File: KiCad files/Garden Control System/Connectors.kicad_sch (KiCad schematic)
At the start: 8 parts, among them J2 PJ-102AH, J3 Debug, J4 USB_C_Receptacle_USB2.0, J5 PJ-102AH, J6 PJ-102AH, J7 PJ-102AH

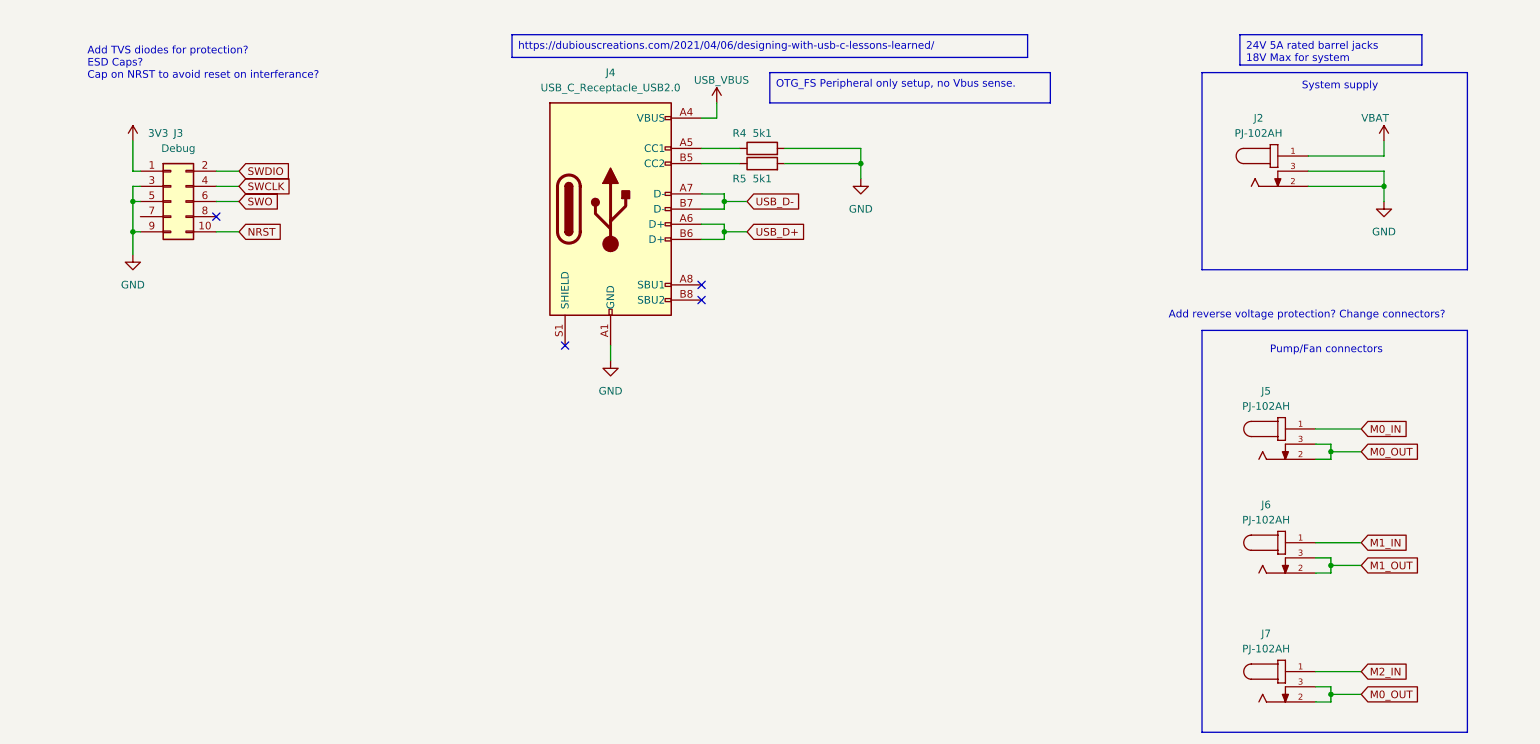
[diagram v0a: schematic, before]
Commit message: we cookin' again. Added LSD and start temp sense section.
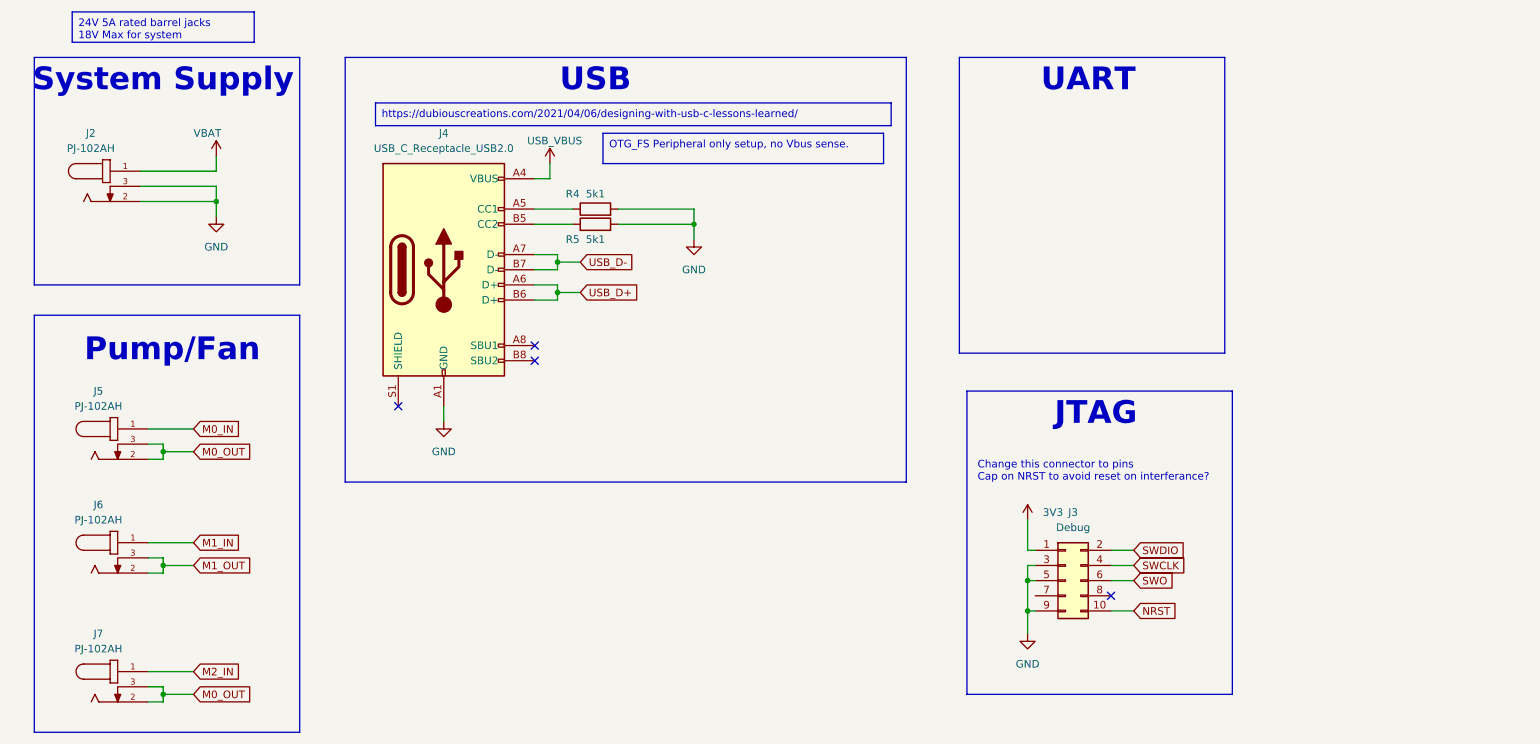
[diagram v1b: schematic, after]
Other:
- note added: "Change this connector to pins Cap on NRST to avoid reset on interferance?"
- note added: "JTAG"
- note added: "Pump/Fan"
- note added: "System Supply"
- note added: "UART"
- note added: "USB"
- note removed: "Add TVS diodes for protection? ESD Caps? Cap on NRST to avoid reset on interferance?"
- note removed: "Add reverse voltage protection? Change connectors?"
- note removed: "Pump/Fan connectors"
- note removed: "System supply"
- moved on the sheet: J2, J3, J4, J5, J6, J7, R4, R5
